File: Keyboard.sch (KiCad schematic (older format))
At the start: 1 part

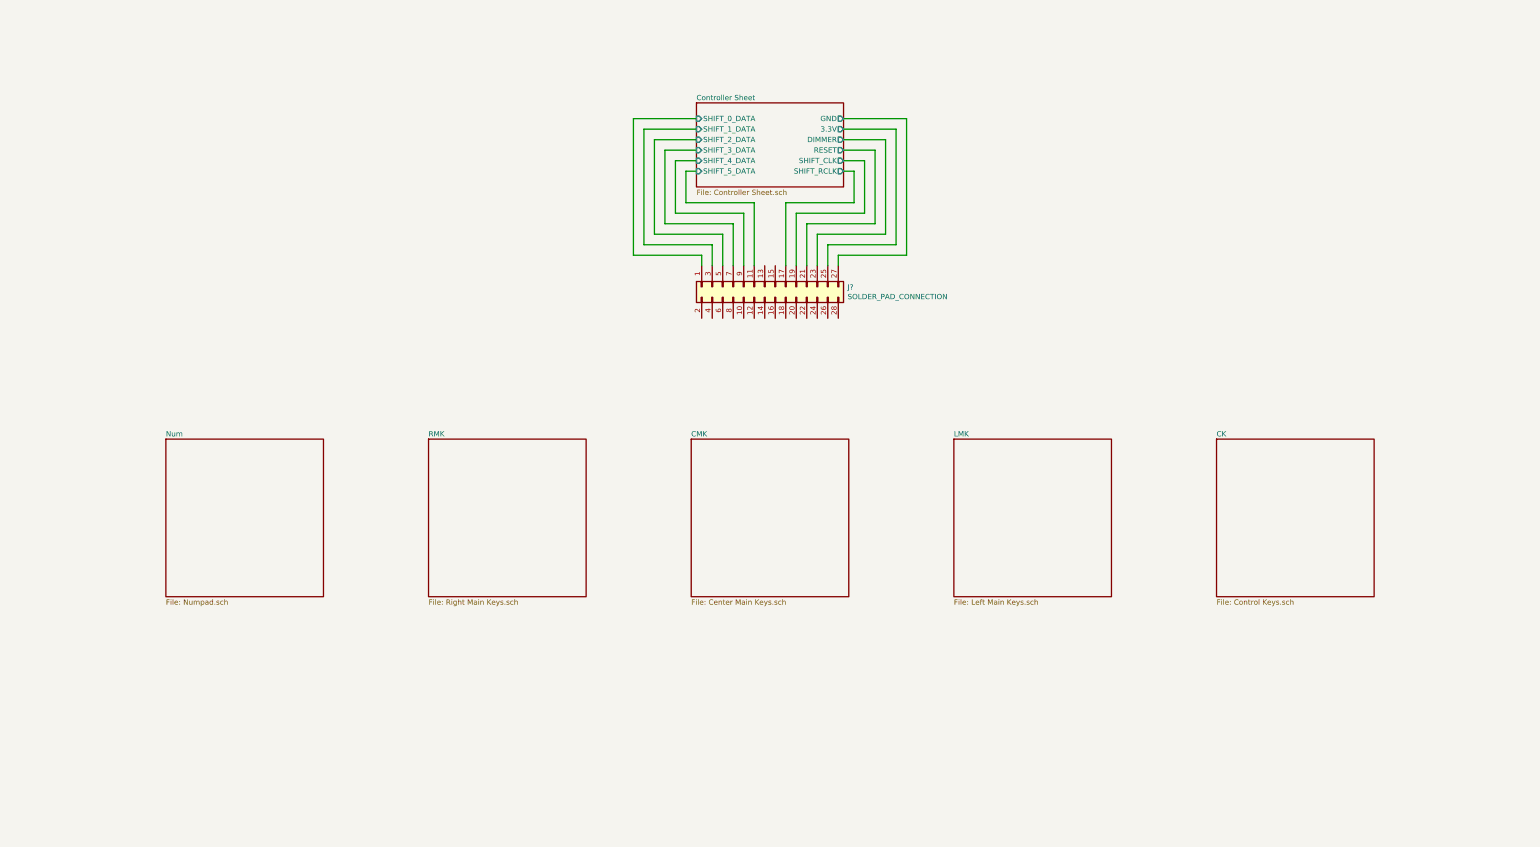
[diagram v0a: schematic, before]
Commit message: 3 Board Schematics Complete
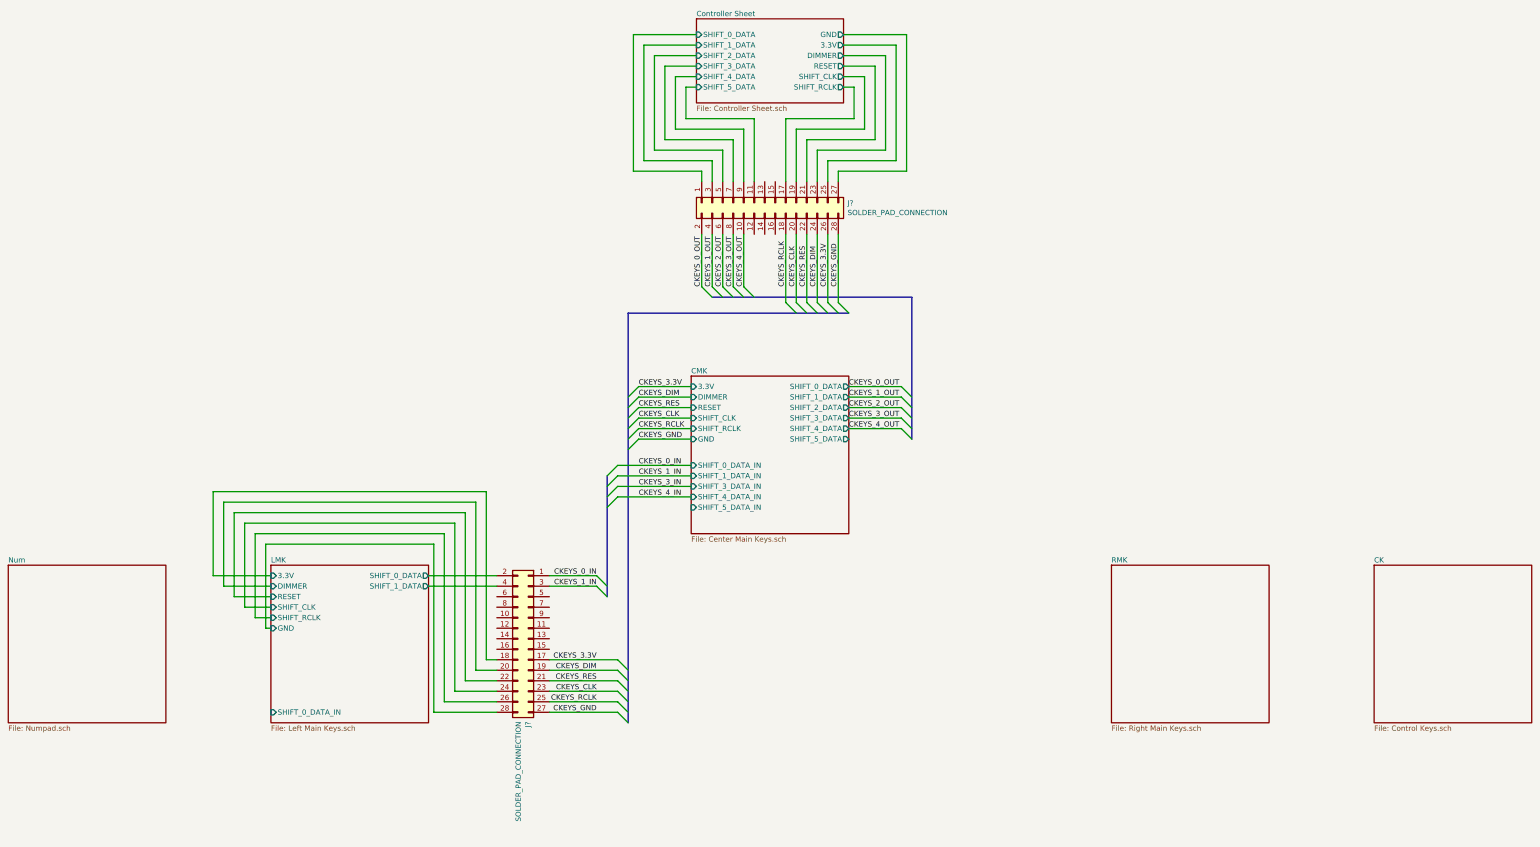
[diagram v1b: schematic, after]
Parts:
- added J?: SOLDER_PAD_CONNECTION, symbol Connector_Generic:Conn_02x14_Odd_Even
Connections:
- net CKEYS_4_OUT: now reaches J?.10 (Pin_10)
- net CKEYS_RCLK: now reaches J?.18 (Pin_18)
- net CKEYS_RCLK: now also J?.25 (Pin_25)
- net CKEYS_0_OUT: now reaches J?.2 (Pin_2)
- net CKEYS_CLK: now reaches J?.20 (Pin_20)
- net CKEYS_CLK: now also J?.23 (Pin_23)
- net CKEYS_RES: now reaches J?.22 (Pin_22)
- net CKEYS_RES: now also J?.21 (Pin_21)
- net CKEYS_DIM: now reaches J?.24 (Pin_24)
- net CKEYS_DIM: now also J?.19 (Pin_19)
- net CKEYS_3.3V: now reaches J?.26 (Pin_26)
- net CKEYS_3.3V: now also J?.17 (Pin_17)
- net CKEYS_GND: now reaches J?.28 (Pin_28)
- net CKEYS_GND: now also J?.27 (Pin_27)
- net CKEYS_1_OUT: now reaches J?.4 (Pin_4)
- net CKEYS_2_OUT: now reaches J?.6 (Pin_6)
- net CKEYS_3_OUT: now reaches J?.8 (Pin_8)
- new net CKEYS_0_IN: J?.1 (Pin_1)
- new net CKEYS_1_IN: J?.3 (Pin_3)
- new net LMK/3.3V: J?.18 (Pin_18)
- new net LMK/DIMMER: J?.20 (Pin_20)
- new net LMK/GND: J?.28 (Pin_28)
- new net LMK/RESET: J?.22 (Pin_22)
- new net LMK/SHIFT_0_DATA: J?.2 (Pin_2)
- new net LMK/SHIFT_1_DATA: J?.4 (Pin_4)
- new net LMK/SHIFT_CLK: J?.24 (Pin_24)
- new net LMK/SHIFT_RCLK: J?.26 (Pin_26)
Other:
- moved on the sheet: J?
